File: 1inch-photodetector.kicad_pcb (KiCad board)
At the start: 4 copper layers, 25.4 x 25.4 mm, 23 parts, among them J1 Conn_01x03, J2 Conn_Coaxial, U1 ADA4898-2, U2 LT3032IDE-12

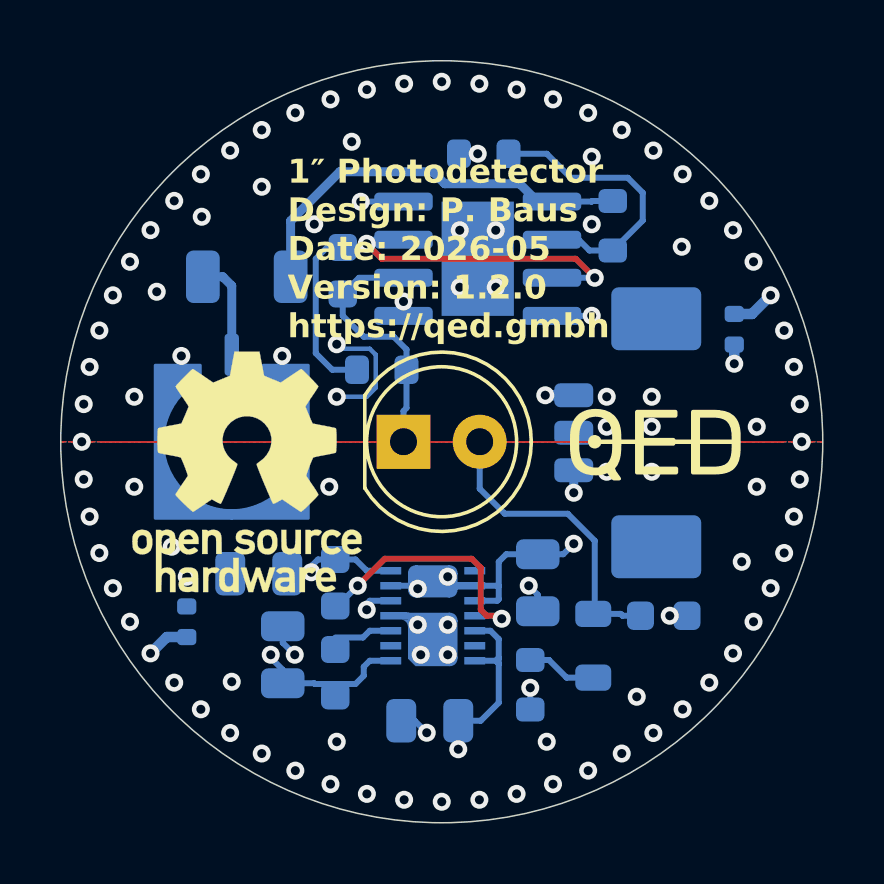
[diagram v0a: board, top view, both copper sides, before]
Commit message: Update components
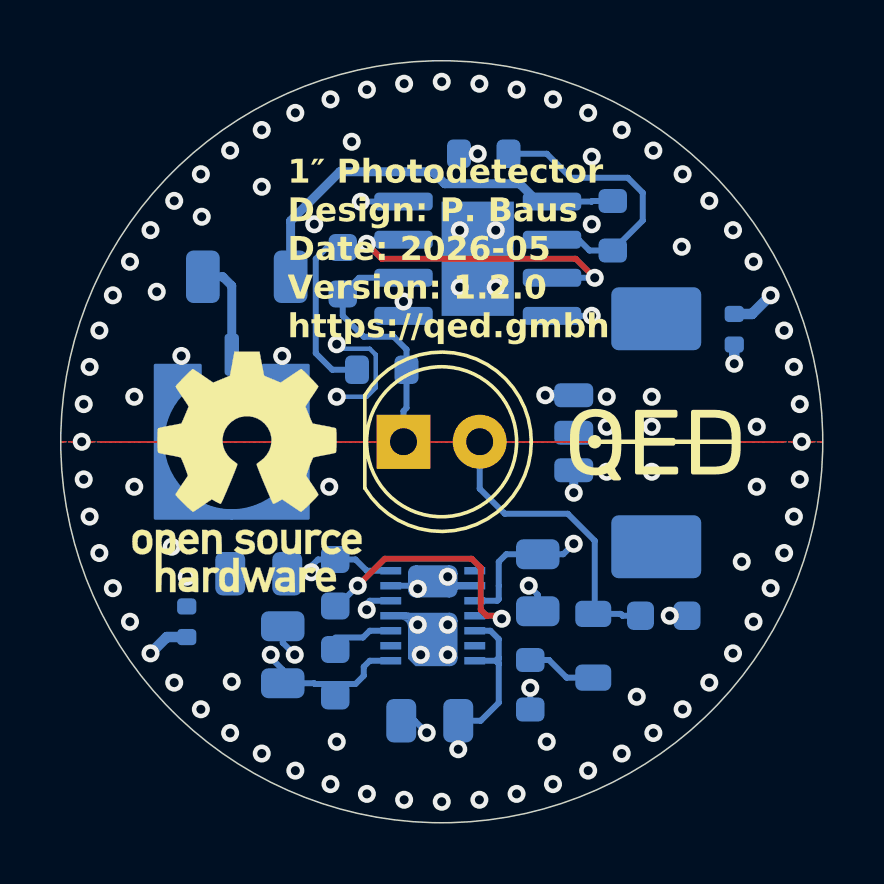
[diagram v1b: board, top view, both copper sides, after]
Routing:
- net /V-: track 8.77 -> 6.72 mm
